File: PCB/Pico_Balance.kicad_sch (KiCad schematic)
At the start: 36 parts, among them J1 XT60PW-M, Q1 NMOS, U1 BMI160, U2 DRV8876PWPR, U3 DRV8876PWPR, U4 LM74610QDGKRQ1, U5 LMR51430

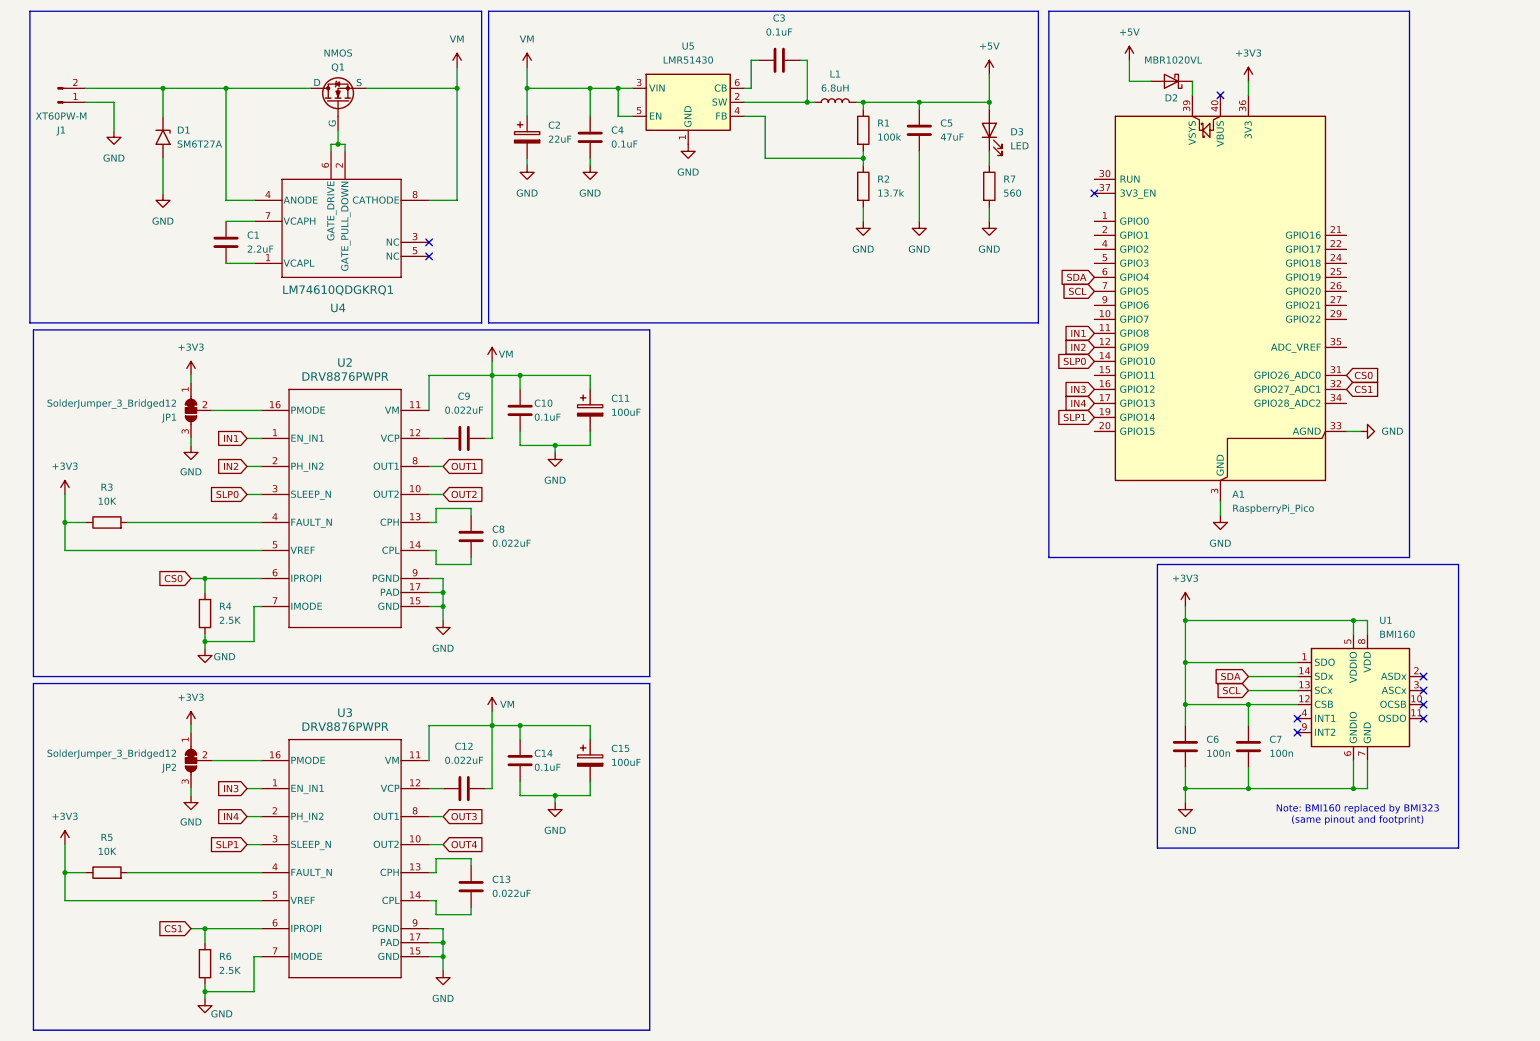
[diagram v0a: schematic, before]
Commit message: Footprint Assignment
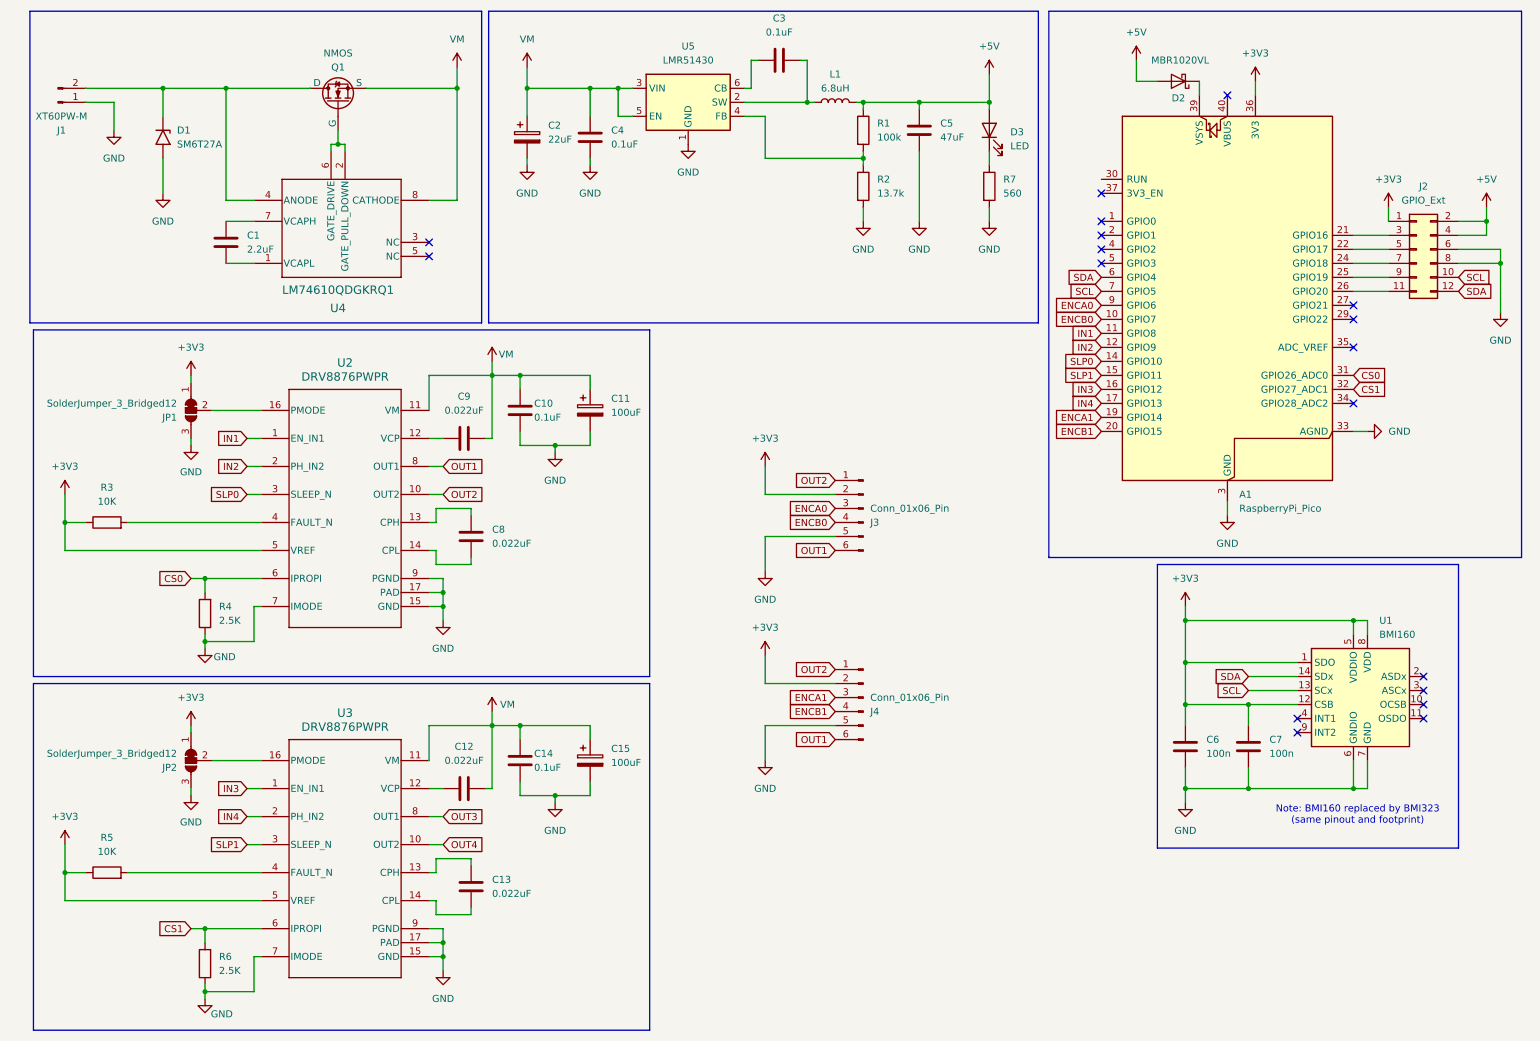
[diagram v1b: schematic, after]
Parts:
- added J2: GPIO_Ext, Connector_PinHeader_2.54mm:PinHeader_2x06_P2.54mm_Vertical, symbol Connector_Generic:Conn_02x06_Odd_Even
- added J3, J4: Conn_01x06_Pin, Connector_PinSocket_2.54mm:PinSocket_1x06_P2.54mm_Vertical, symbol Connector:Conn_01x06_Pin
- C1: footprint (none) -> Capacitor_SMD:C_1206_3216Metric
- C10, C12, C13, C14, C3, C4, C6, C7, C8, C9: footprint (none) -> Capacitor_SMD:C_0603_1608Metric
- C11, C15: footprint (none) -> Capacitor_SMD:CP_Elec_10x10.5
- C2: footprint (none) -> Capacitor_SMD:CP_Elec_5x5.4
- C5: footprint (none) -> Capacitor_SMD:C_1210_3225Metric
- L1: footprint (none) -> Inductor_SMD:L_APV_APH0630
- R1, R2, R3, R4, R5, R6, R7: footprint (none) -> Resistor_SMD:R_0603_1608Metric
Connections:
- net +3V3: now also J2.1 (Pin_1), J3.2 (Pin_2), J4.2 (Pin_2)
- net +5V: now also J2.2 (Pin_2), J2.4 (Pin_4)
- net GND: now also J2.6 (Pin_6), J2.8 (Pin_8), J3.5 (Pin_5), J4.5 (Pin_5)
- net OUT1: now also J3.6 (Pin_6), J4.6 (Pin_6)
- net OUT2: now also J3.1 (Pin_1), J4.1 (Pin_1)
- net SCL: now also J2.10 (Pin_10)
- net SDA: now also J2.12 (Pin_12)
- net SLP1: now also A1.15 (GPIO11); no longer A1.19 (GPIO14)
- net ENCB0: now reaches A1.10 (GPIO7)
- net ENCB0: now also J3.4 (Pin_4)
- net ENCB1: now reaches A1.20 (GPIO15)
- net ENCB1: now also J4.4 (Pin_4)
- net at A1.21 (GPIO16): now also J2.3 (Pin_3)
- net at A1.22 (GPIO17): now also J2.5 (Pin_5)
- net at A1.24 (GPIO18): now also J2.7 (Pin_7)
- net at A1.25 (GPIO19): now also J2.9 (Pin_9)
- net at A1.26 (GPIO20): now also J2.11 (Pin_11)
- net ENCA0: now reaches A1.9 (GPIO6)
- net ENCA0: now also J3.3 (Pin_3)
- new net ENCA1: A1.19 (GPIO14), J4.3 (Pin_3)
- no-connect marks 10 -> 18
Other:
- moved on the sheet: A1, D2

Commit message: Very Initial Layout and footprint updates
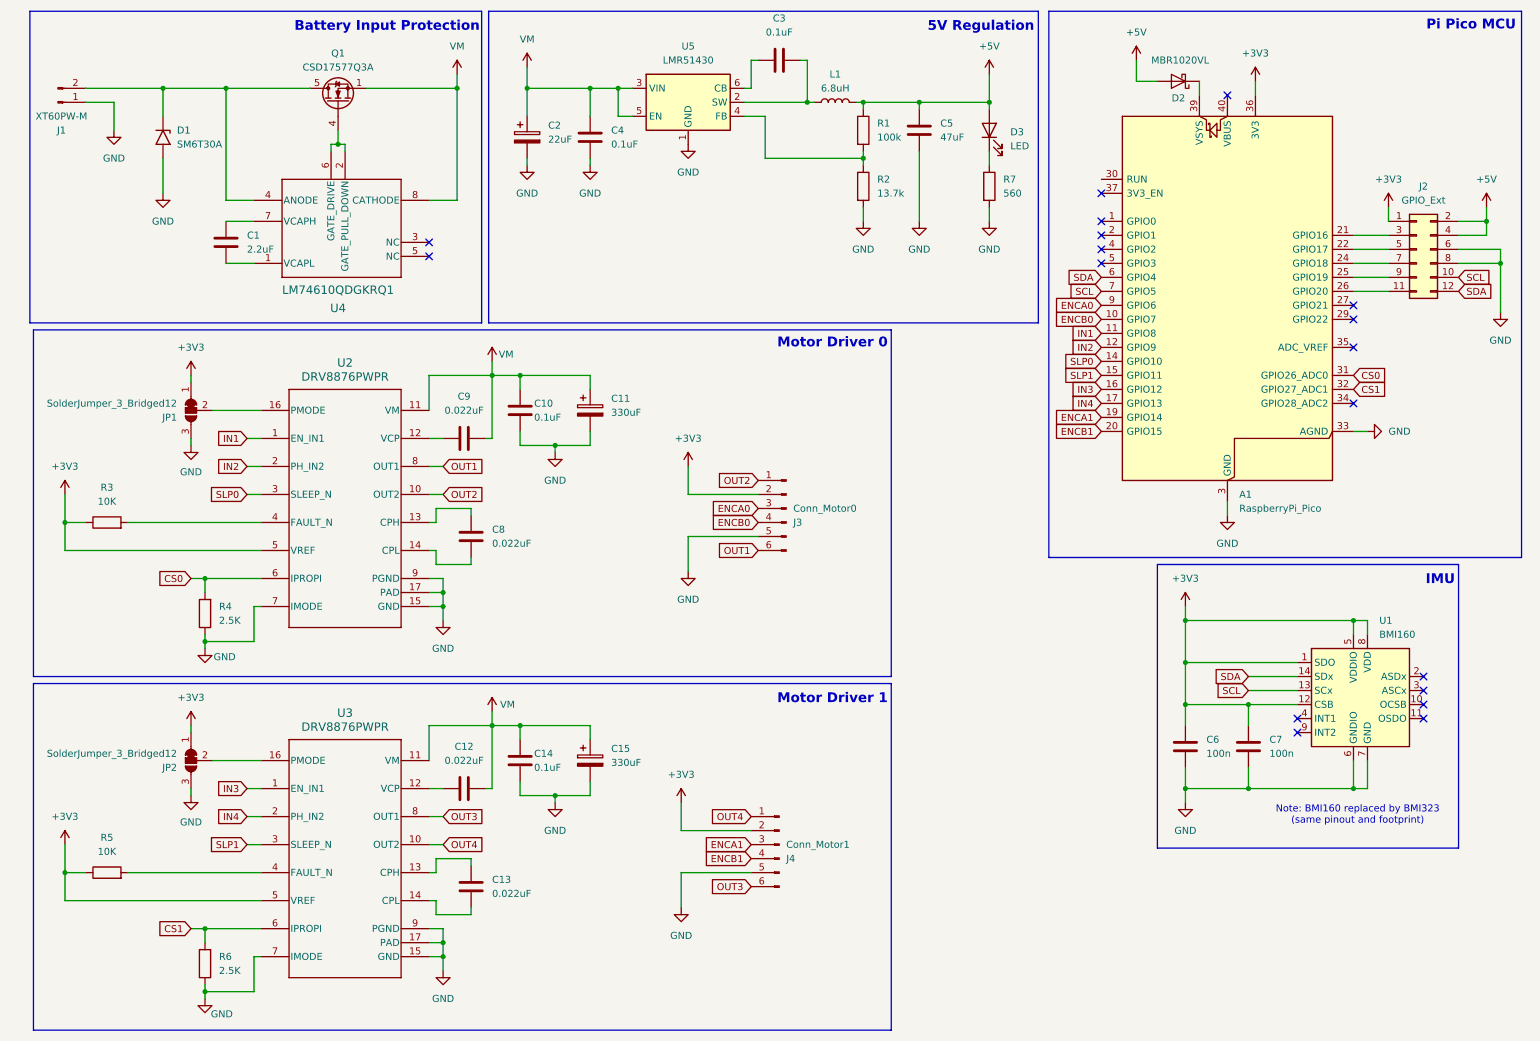
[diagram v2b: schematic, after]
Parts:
- removed Q1: NMOS, Package_SO:SO-8_3.9x4.9mm_P1.27mm, symbol Simulation_SPICE:NMOS
- added Q1: CSD17577Q3A, Package_SON:VSON-8_3.3x3.3mm_P0.65mm_NexFET, symbol Transistor_FET:CSD17577Q3A
- C11, C15: value 100uF -> 330uF
- D1: value SM6T27A -> SM6T30A; footprint LED_SMD:LED-L1T2_LUMILEDS -> Diode_SMD:D_SMB
- J3: value Conn_01x06_Pin -> Conn_Motor0
- J4: value Conn_01x06_Pin -> Conn_Motor1
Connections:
- net OUT1: no longer J4.6 (Pin_6)
- net OUT2: no longer J4.1 (Pin_1)
- net OUT3: now also J4.6 (Pin_6)
- net OUT4: now also J4.1 (Pin_1)
- net VM: now also Q1.1 (S), Q1.2 (S), Q1.3 (S)
- net at D1.1 (A1), J1.2 (Pin_2), U4.4 (ANODE): now also Q1.5 (D)
- net at U4.2 (GATE_PULL_DOWN), U4.6 (GATE_DRIVE): now also Q1.4 (G)
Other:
- note added: "5V Regulation"
- note added: "Battery Input Protection"
- note added: "IMU"
- note added: "Motor Driver 0"
- note added: "Motor Driver 1"
- note added: "Pi Pico MCU"
- moved on the sheet: J3, J4
